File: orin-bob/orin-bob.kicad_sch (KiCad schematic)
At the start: 0 parts

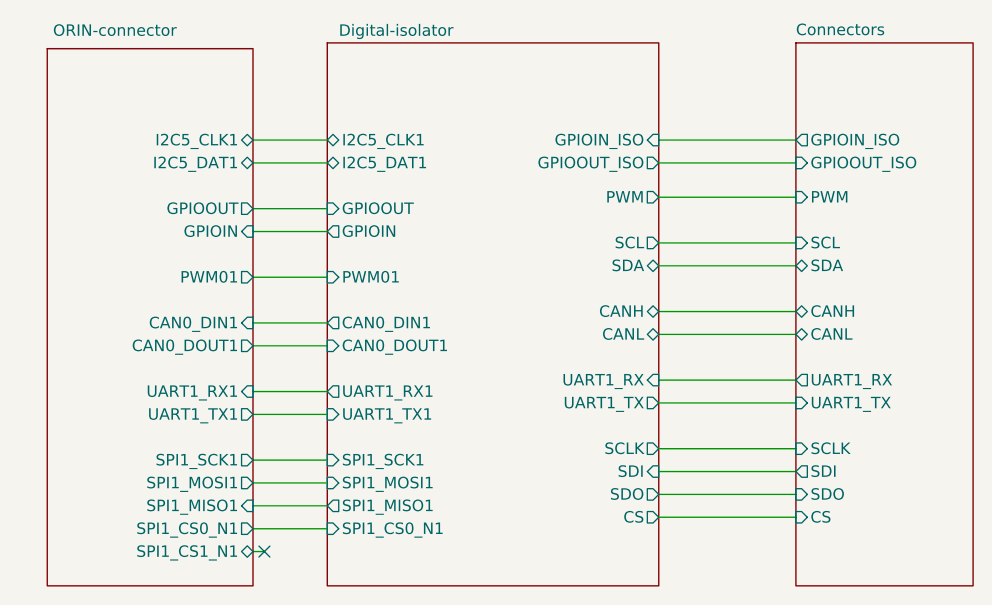
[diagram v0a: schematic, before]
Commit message: Finished: Orin-BoB
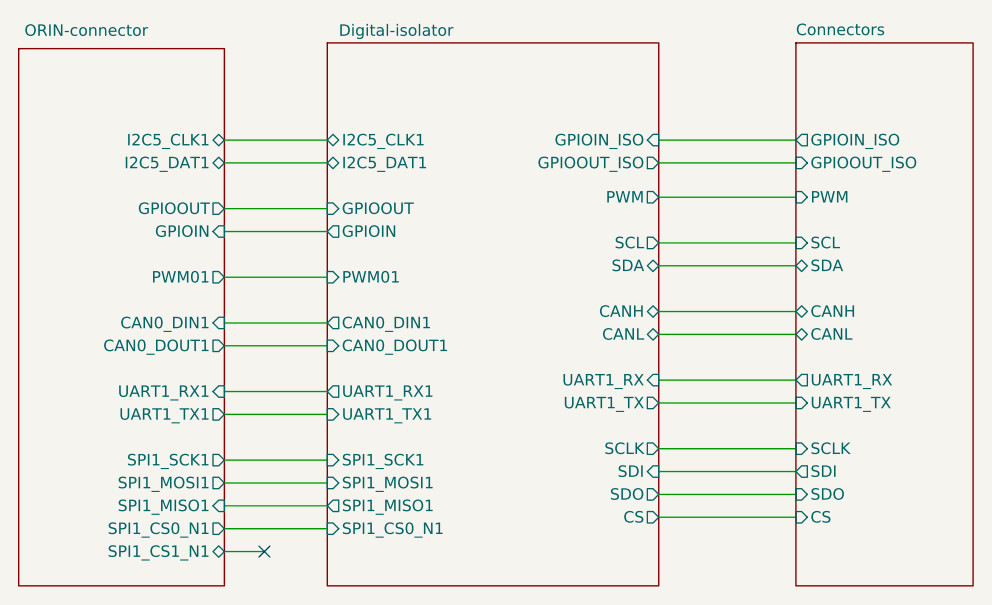
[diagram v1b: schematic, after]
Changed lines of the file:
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@@
 	(wire
 		(pts
-			(xy 71.755 64.77) (xy 80.01 64.77)
-		)
-		(stroke
-			(width 0)
-			(type default)
-		)
-	)
-	(wire
-		(pts
-			(xy 71.755 69.85) (xy 80.01 69.85)
+			(xy 68.58 64.77) (xy 80.01 64.77)
+		)
+		(stroke
+			(width 0)
+			(type default)
+		)
+	)
+	(wire
+		(pts
+			(xy 68.58 69.85) (xy 80.01 69.85)
 		)
 		(stroke
@@
 	(wire
 		(pts
-			(xy 71.755 85.09) (xy 80.01 85.09)
+			(xy 68.58 85.09) (xy 80.01 85.09)
 		)
 		(stroke
@@
 	(wire
 		(pts
-			(xy 71.755 77.47) (xy 80.01 77.47)
+			(xy 68.58 77.47) (xy 80.01 77.47)
 		)
 		(stroke
@@
 	(wire
 		(pts
-			(xy 71.755 82.55) (xy 80.01 82.55)
-		)
-		(stroke
-			(width 0)
-			(type default)
-		)
-	)
-	(wire
-		(pts
-			(xy 71.755 87.63) (xy 73.025 87.63)
-		)
-		(stroke
-			(width 0)
-			(type default)
-		)
-	)
-	(wire
-		(pts
-			(xy 71.755 52.07) (xy 80.01 52.07)
+			(xy 68.58 82.55) (xy 80.01 82.55)
+		)
+		(stroke
+			(width 0)
+			(type default)
+		)
+	)
+	(wire
+		(pts
+			(xy 68.58 87.63) (xy 73.025 87.63)
+		)
+		(stroke
+			(width 0)
+			(type default)
+		)
+	)
+	(wire
+		(pts
+			(xy 68.58 52.07) (xy 80.01 52.07)
 		)
 		(stroke
@@
 	(wire
 		(pts
-			(xy 71.755 80.01) (xy 80.01 80.01)
-		)
-		(stroke
-			(width 0)
-			(type default)
-		)
-	)
-	(wire
-		(pts
-			(xy 71.755 41.91) (xy 80.01 41.91)
+			(xy 68.58 80.01) (xy 80.01 80.01)
+		)
+		(stroke
+			(width 0)
+			(type default)
+		)
+	)
+	(wire
+		(pts
+			(xy 68.58 41.91) (xy 80.01 41.91)
 		)
 		(stroke
@@
 	(wire
 		(pts
-			(xy 71.755 49.53) (xy 80.01 49.53)
+			(xy 68.58 49.53) (xy 80.01 49.53)
 		)
 		(stroke
@@
 	(wire
 		(pts
-			(xy 71.755 57.15) (xy 80.01 57.15)
+			(xy 68.58 57.15) (xy 80.01 57.15)
 		)
 		(stroke
@@
 	(wire
 		(pts
-			(xy 71.755 62.23) (xy 80.01 62.23)
-		)
-		(stroke
-			(width 0)
-			(type default)
-		)
-	)
-	(wire
-		(pts
-			(xy 71.755 72.39) (xy 80.01 72.39)
-		)
-		(stroke
-			(width 0)
-			(type default)
-		)
-	)
-	(wire
-		(pts
-			(xy 71.755 44.45) (xy 80.01 44.45)
+			(xy 68.58 62.23) (xy 80.01 62.23)
+		)
+		(stroke
+			(width 0)
+			(type default)
+		)
+	)
+	(wire
+		(pts
+			(xy 68.58 72.39) (xy 80.01 72.39)
+		)
+		(stroke
+			(width 0)
+			(type default)
+		)
+	)
+	(wire
+		(pts
+			(xy 68.58 44.45) (xy 80.01 44.45)
 		)
 		(stroke
@@
 	)
 	(sheet
-		(at 48.895 31.75)
+		(at 45.72 31.75)
 		(size 22.86 59.69)
 		(exclude_from_sim no)
@@
 		)
 		(property "Sheetname" "ORIN-connector"
-			(at 49.53 30.48 0)
+			(at 46.355 30.48 0)
 			(show_name no)
 			(do_not_autoplace no)
@@
 		)
 		(property "Sheetfile" "orin-connector.kicad_sch"
-			(at 48.895 66.3706 0)
+			(at 45.72 66.3706 0)
 			(hide yes)
 			(show_name no)
@@
 		)
 		(pin "CAN0_DIN1" input
-			(at 71.755 62.23 0)
+			(at 68.58 62.23 0)
 			(effects
 				(font
@@
 		)
 		(pin "CAN0_DOUT1" output
-			(at 71.755 64.77 0)
+			(at 68.58 64.77 0)
 			(effects
 				(font
@@
 		)
 		(pin "I2C5_CLK1" bidirectional
-			(at 71.755 41.91 0)
+			(at 68.58 41.91 0)
 			(effects
 				(font
@@
 		)
 		(pin "I2C5_DAT1" bidirectional
-			(at 71.755 44.45 0)
+			(at 68.58 44.45 0)
 			(effects
 				(font
@@
 		)
 		(pin "SPI1_CS0_N1" output
-			(at 71.755 85.09 0)
+			(at 68.58 85.09 0)
 			(effects
 				(font
@@
 		)
 		(pin "SPI1_CS1_N1" bidirectional
-			(at 71.755 87.63 0)
+			(at 68.58 87.63 0)
 			(effects
 				(font
@@
 		)
 		(pin "SPI1_MISO1" input
-			(at 71.755 82.55 0)
+			(at 68.58 82.55 0)
 			(effects
 				(font
@@
 		)
 		(pin "SPI1_MOSI1" output
-			(at 71.755 80.01 0)
+			(at 68.58 80.01 0)
 			(effects
 				(font
@@
 		)
 		(pin "SPI1_SCK1" output
-			(at 71.755 77.47 0)
+			(at 68.58 77.47 0)
 			(effects
 				(font
@@
 		)
 		(pin "UART1_RX1" input
-			(at 71.755 69.85 0)
+			(at 68.58 69.85 0)
 			(effects
 				(font
@@
 		)
 		(pin "UART1_TX1" output
-			(at 71.755 72.39 0)
+			(at 68.58 72.39 0)
 			(effects
 				(font
@@
 		)
 		(pin "GPIOOUT" output
-			(at 71.755 49.53 0)
+			(at 68.58 49.53 0)
 			(effects
 				(font
@@
 		)
 		(pin "PWM01" output
-			(at 71.755 57.15 0)
+			(at 68.58 57.15 0)
 			(effects
 				(font
@@
 		)
 		(pin "GPIOIN" input
-			(at 71.755 52.07 0)
-			(effects
-				(font
+			(at 68.58 52.07 0)
+			(effects
+				(font
